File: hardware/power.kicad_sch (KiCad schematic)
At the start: 67 parts, among them J2 Conn_01x03, U32 LDK220M-R, U33 PAC1934x-xJQ, U34 LDK220M-R, U37 PM8903A, U39 NCV8187AMLExCG, U40 NCV8187AMLExCG

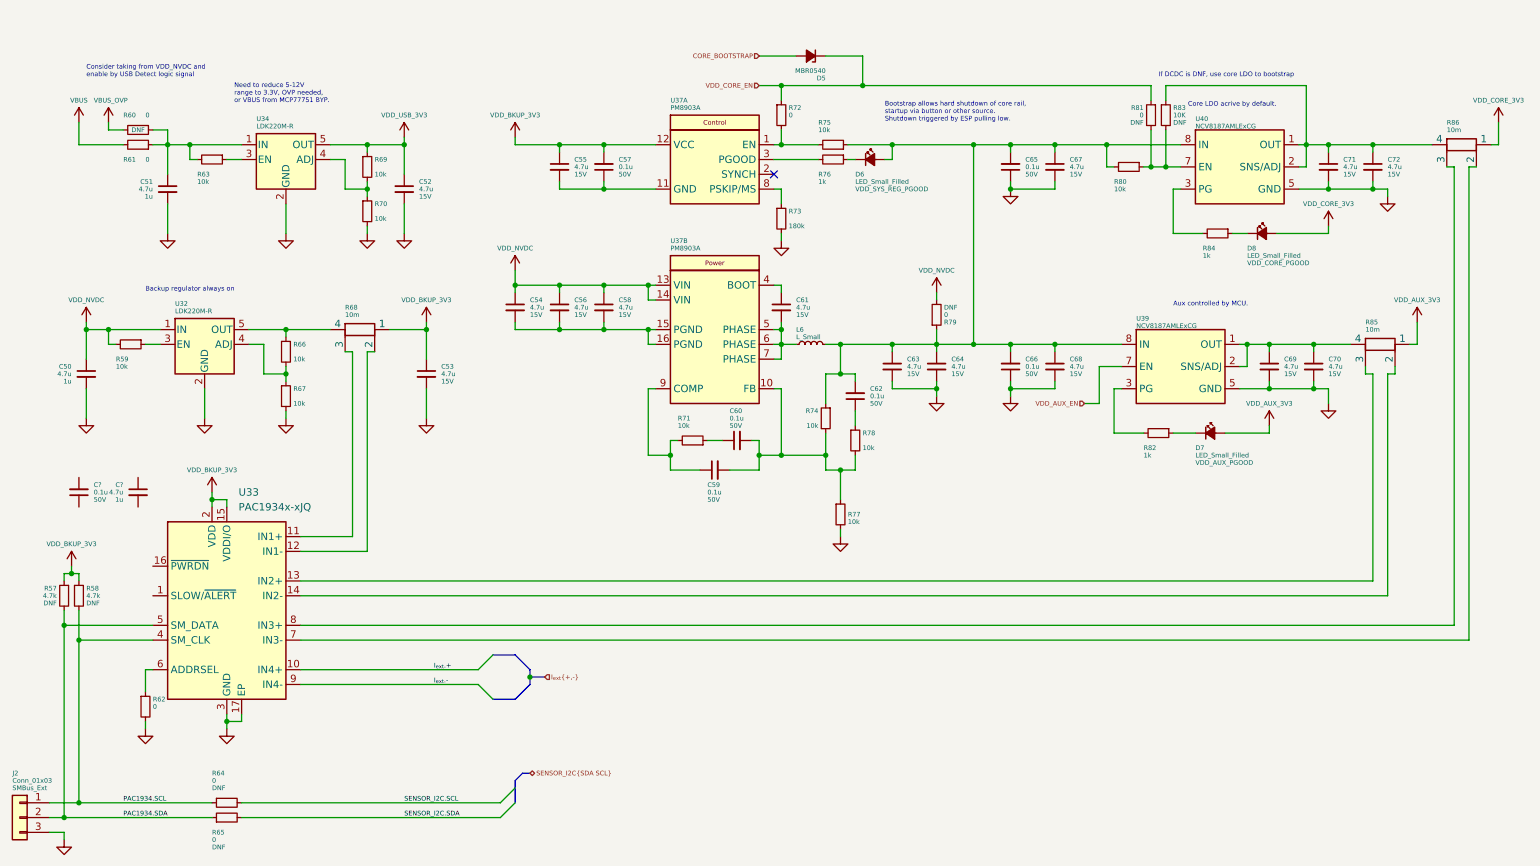
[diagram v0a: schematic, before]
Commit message: hardware update
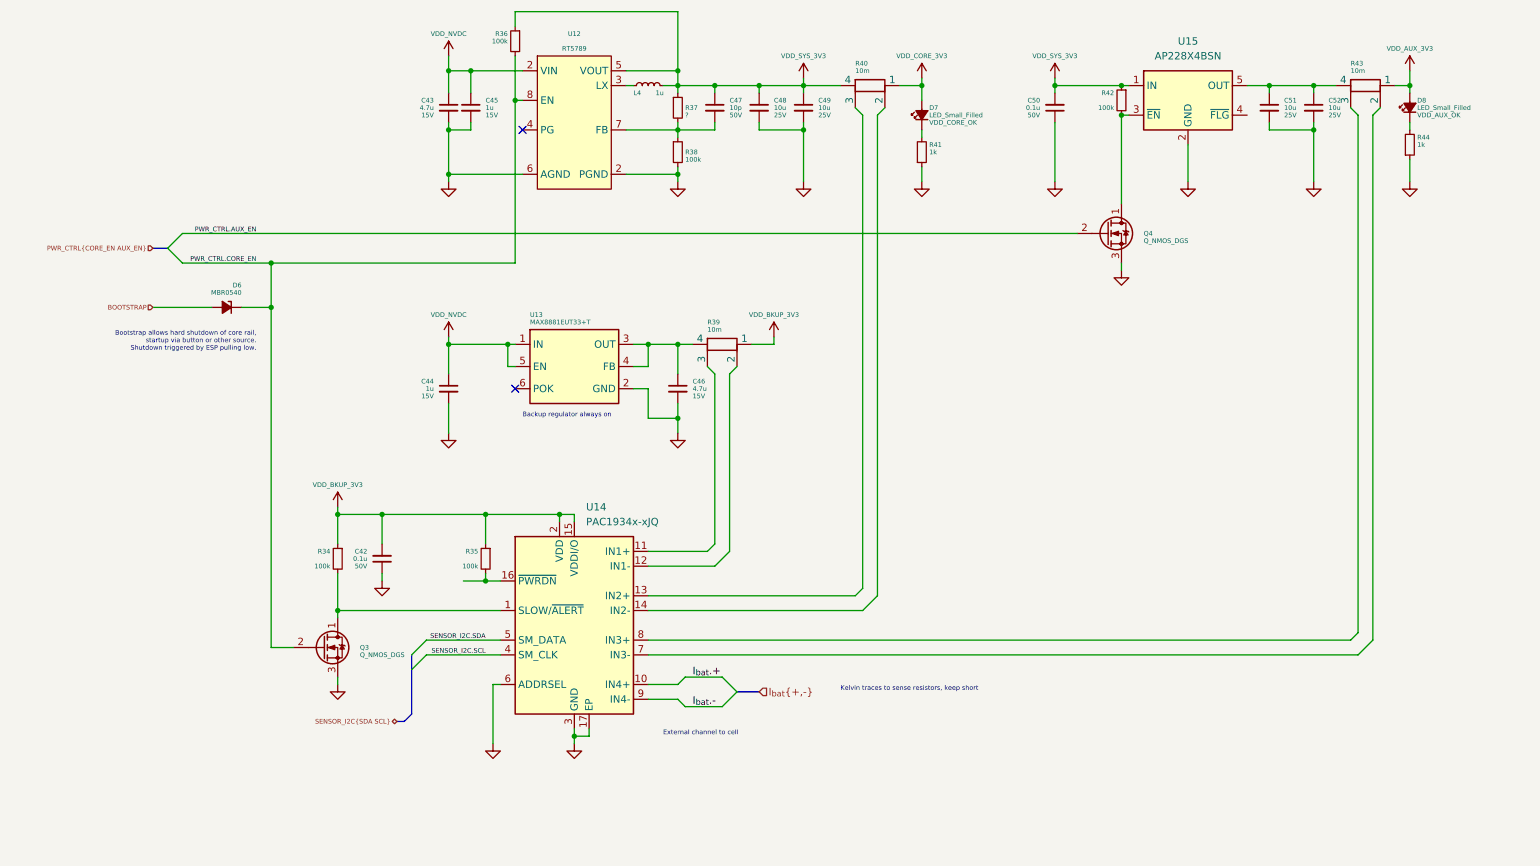
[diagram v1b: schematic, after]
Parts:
- removed C53, C54, C55, C56, C58, C61, C63, C64, C67, C68, C69, C70, C71, C72, C?: 4.7u, Capacitor_SMD:C_0603_1608Metric, symbol Device:C_Small
- removed C57, C59, C60, C62, C65, C66: 0.1u, Capacitor_SMD:C_0603_1608Metric, symbol Device:C_Small
- removed D5: MBR0540, Diode_SMD:D_0603_1608Metric, symbol Device:D_Zener_Small_Filled
- removed D6: LED_Small_Filled, LED_SMD:LED_0603_1608Metric, symbol Device:LED_Small_Filled
- removed J2: Conn_01x03, Connector_PinHeader_1.00mm:PinHeader_1x03_P1.00mm_Vertical, symbol Connector_Generic:Conn_01x03
- removed L6: L_Small, Inductor_SMD:L_Bourns-SRN4018, symbol Device:L_Small
- removed R57, R58: 4.7k, Resistor_SMD:R_0603_1608Metric, symbol Device:R_Small
- removed R59, R63, R66, R67, R69, R70, R71, R74, R77, R78, R80: 10k, Resistor_SMD:R_0603_1608Metric, symbol Device:R_Small
- removed R60, R61, R62, R64, R65, R72, R79, R81: 0, Resistor_SMD:R_0603_1608Metric, symbol Device:R_Small
- removed R73: 180k, Resistor_SMD:R_0603_1608Metric, symbol Device:R_Small
- removed R76, R82, R84: 1k, Resistor_SMD:R_0603_1608Metric, symbol Device:R_Small
- removed R83: 10K, Resistor_SMD:R_0603_1608Metric, symbol Device:R_Small
- removed R85, R86: 10m, Resistor_SMD:R_1210_3225Metric, symbol Device:R_Shunt
- removed U32, U34: LDK220M-R, Package_TO_SOT_SMD:SOT-23-5, symbol Regulator_Linear:LDK130-ADJ_SOT23_SOT353
- removed U37: PM8903A, Package_DFN_QFN:VQFN-16-1EP_3x3mm_P0.5mm_EP1.45x1.45mm_ThermalVias, symbol bt_PMIC_DCDC_Buck:PM8903A
- removed U39, U40: NCV8187AMLExCG, Package_DFN_QFN:DFN-8-1EP_3x3mm_P0.65mm_EP1.55x2.4mm, symbol bt_PMIC_Linear:NCV8187AMLExCG
- added C43, C46: 4.7u, Capacitor_SMD:C_0603_1608Metric, symbol Device:C_Small
- added C45: 1u, Capacitor_SMD:C_0603_1608Metric, symbol Device:C_Small
- added C47: 10p, Capacitor_SMD:C_0402_1005Metric, symbol Device:C_Small
- added C48, C49: 10u, Capacitor_SMD:C_0805_2012Metric, symbol Device:C_Small
- added C50: 0.1u, Capacitor_SMD:C_0402_1005Metric, symbol Device:C_Small
- added D6: MBR0540, LED_SMD:LED_0603_1608Metric, symbol Device:D_Zener_Small_Filled
- added L4: 1u, Inductor_SMD:L_Wuerth_MAPI-2510, symbol Device:L_Small
- added Q3, Q4: Q_NMOS_DGS, Package_TO_SOT_SMD:SOT-323_SC-70, symbol Device:Q_NMOS_DGS
- added R34, R35, R38, R42: 100k, Resistor_SMD:R_0402_1005Metric, symbol Device:R_Small
- added R37: ?, Resistor_SMD:R_0402_1005Metric, symbol Device:R_Small
- added R40: 10m, Resistor_SMD:R_0603_1608Metric_Pad0.98x0.95mm_HandSolder, symbol Device:R_Shunt
- added R41, R44: 1k, Resistor_SMD:R_0402_1005Metric, symbol Device:R_Small
- added R43: 10m, Resistor_SMD:R_0603_1608Metric, symbol Device:R_Shunt
- added U12: RT5789, Package_DFN_QFN:DFN-10-1EP_3x3mm_P0.5mm_EP1.55x2.48mm, symbol bt_PMIC_DCDC_Buck:RT5789
- added U13: MAX8881EUT33+T, Package_TO_SOT_SMD:SOT-23-6, symbol bt_PMIC_Linear:MAX8881EUT33+T
- added U15: AP228X4BSN, bt_Package_DFN:Diodes_UDFN2020-6, symbol bt_Power_Management:AP228X4BSN
- C42: renamed from C?; footprint Capacitor_SMD:C_0603_1608Metric -> Capacitor_SMD:C_0402_1005Metric
- C44: renamed from C50; value 4.7u -> 1u; Voltage 1u -> 15V
- C51: value 4.7u -> 10u; footprint Capacitor_SMD:C_0603_1608Metric -> Capacitor_SMD:C_0805_2012Metric; Voltage 1u -> 25V
- C52: value 4.7u -> 10u; footprint Capacitor_SMD:C_0603_1608Metric -> Capacitor_SMD:C_0805_2012Metric; Voltage 15V -> 25V
- D7: Label VDD_AUX_PGOOD -> VDD_CORE_OK
- D8: Label VDD_CORE_PGOOD -> VDD_AUX_OK
- R36: renamed from R75; value 10k -> 100k; footprint Resistor_SMD:R_0603_1608Metric -> Resistor_SMD:R_0402_1005Metric
- R39: renamed from R68; footprint Resistor_SMD:R_1210_3225Metric -> Resistor_SMD:R_0603_1608Metric_Pad0.98x0.95mm_HandSolder
- renumbered U33 to U14
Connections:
- net PAC1934.SCL is gone; now on net SENSOR_I2C.SCL: U14.4 (SM_CLK)
- net PAC1934.SDA is gone; now on net SENSOR_I2C.SDA: U14.5 (SM_DATA)
- net VDD_USB_3V3 is gone; now on an unnamed net: C52.1
- net 3V3_CORE: now also D7.2 (A), R40.1; no longer D8.2 (A)
- net GND: now also C42.1, U14.6 (ADDRSEL), C43.2, C45.2, C46.2, C48.2, C49.2, C50.1, Q3.3 (S), Q4.3 (S), R38.2, R41.1, R44.1, U12.2 (VIN), U12.6 (AGND), U13.2 (GND), U15.2 (GND)
- net VCC_BKUP_3V3: now also C42.2, R34.1, R35.1
- net VDD_AUX_3V3: now also D8.2 (A), R43.1; no longer D7.2 (A)
- net VDD_NVDC: now also C43.1, C45.1, U12.2 (VIN), U13.1 (IN), U13.5 (EN)
- net at D8.1 (K): now also R44.2
- net VDD_SYS_3V3: now reaches R36.1
- net VDD_SYS_3V3: now also C47.1, C48.1, C49.1, C50.2, L4.2, R37.1, R40.4, R42.1, U12.5 (VOUT), U15.1 (IN)
- net PWR_CTRL.CORE_EN: now reaches R36.2
- net PWR_CTRL.CORE_EN: now also D6.1 (K), Q3.2 (G), U12.8 (EN)
- net at R39.4: now also C46.1, U13.3 (OUT), U13.4 (FB)
- net at C51.1: now also R43.4, U15.5 (OUT)
- net at D7.1 (K): now also R41.2
- net at U14.1 (SLOW/~{ALERT}): now also Q3.1 (D), R34.2
- net at U14.13 (IN2+): now also R40.3
- net at U14.14 (IN2-): now also R40.2
- net at U14.16 (~{PWRDN}): now also R35.2
- net at U14.7 (IN3-): now also R43.2
- net at U14.8 (IN3+): now also R43.3
- net I_{ext}.+ renamed I_{bat}.+
- net I_{ext}.- renamed I_{bat}.-
- new net: L4.1, U12.3 (LX)
- new net: Q4.1 (D), R42.2, U15.3 (~{EN})
- new net: C47.2, R37.2, R38.1, U12.7 (FB)
- new net BOOTSTRAP: D6.2 (A)
- new net PWR_CTRL.AUX_EN: Q4.2 (G)
- no-connect marks 1 -> 2
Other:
- note added: "External channel to cell"
- note added: "Kelvin traces to sense resistors, keep short"
- note removed: "Aux controlled by MCU."
- note removed: "Consider taking from VDD_NVDC and enable by USB Detect logic signal"
- note removed: "Core LDO acrive by default."
- note removed: "If DCDC is DNF, use core LDO to bootstrap"
- note removed: "Need to reduce 5-12V range to 3.3V, OVP needed, or VBUS from MCP77751 BYP."
- moved on the sheet: C42, C44, R36, R39, U14
